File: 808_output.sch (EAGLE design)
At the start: 31 parts, among them IC1 TL072P

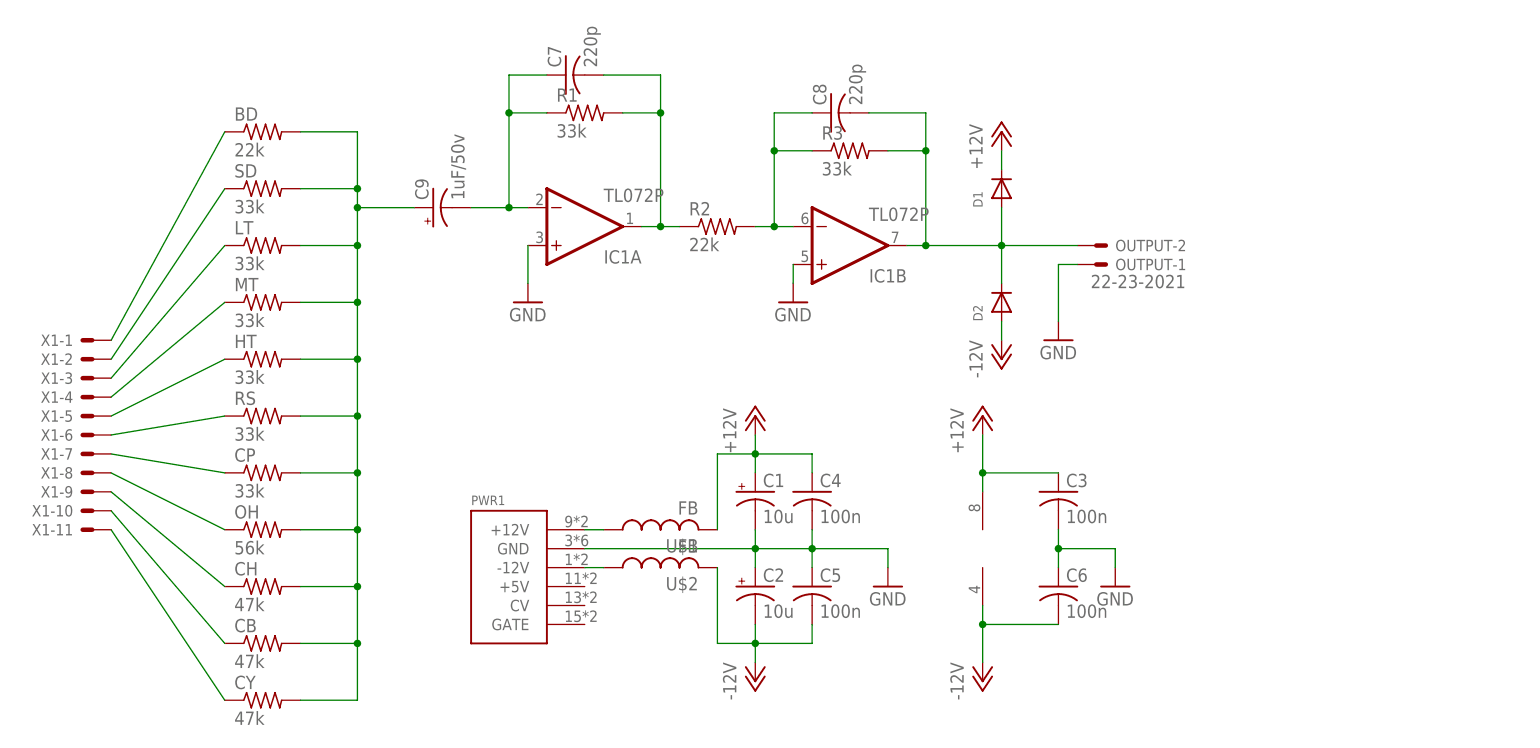
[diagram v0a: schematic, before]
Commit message: closer to og 808
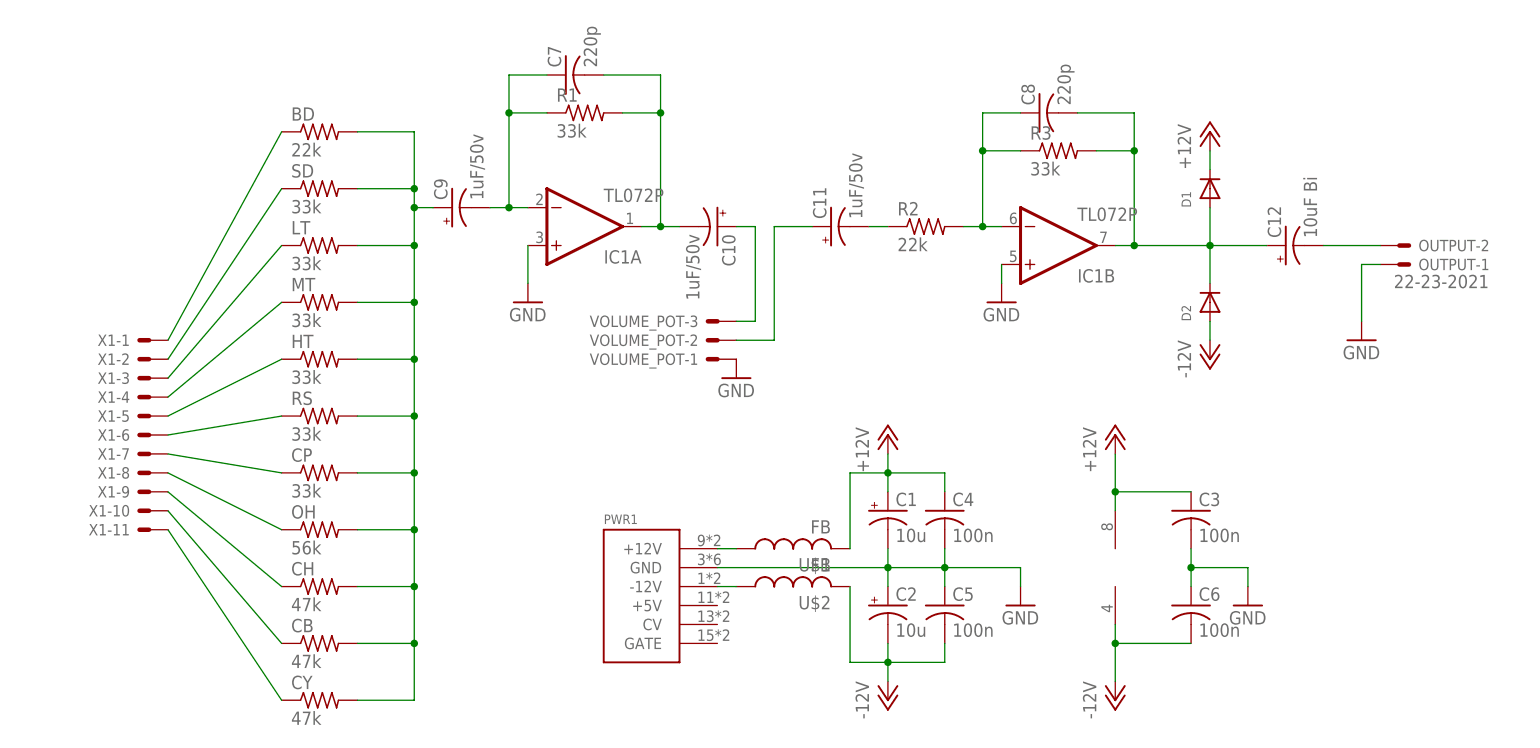
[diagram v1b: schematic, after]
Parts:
- added C10, C11: 1uF/50v, rcl:CPOL-USB45181A
- added C12: 10uF Bi, rcl:CPOL-USB45181A
- added VOLUME_POT: (no value), con-molex:KK-156-3
- C9: device rcl:CPOL-USB45181A -> rcl:CPOL-USB45181B
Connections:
- new net N$18: C11.-, R2.1
- new net N$20: C10.+, VOLUME_POT-3.S
- new net N$21: C11.+, VOLUME_POT-2.S
- new net N$22: C12.-, OUTPUT-2.S
- net GND: now also VOLUME_POT-1.S
- net N$15: now also C10.-; no longer R2.1
- net N$19: now also C12.+; no longer OUTPUT-2.S
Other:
- moved on the sheet: BD, C1, C2, C3, C4, C5, C6, C8, C9, CB, CH, CP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
